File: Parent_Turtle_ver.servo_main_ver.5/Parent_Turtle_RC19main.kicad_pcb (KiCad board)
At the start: 2 copper layers, 70 x 60 mm, 61 parts, among them P1 CONN_02X15, P10 WRITING, P11 A/D, P12 5V_in, P13 CONN_02X04, P14 I/O, P15 CONN_02X04, P16 PWM, P17 SERIAL0, P2 CONN_02X15, P3 CAN, P4 CAN, P5 PWM, P6 SERIAL1, P7 SERIAL2, P8 WRITING_IN, P9 CAN_JP, Q1 NPN, SW1 SW1, SW2 SW0, U1 MAX3051, U2 MCP2221, U3 78L05

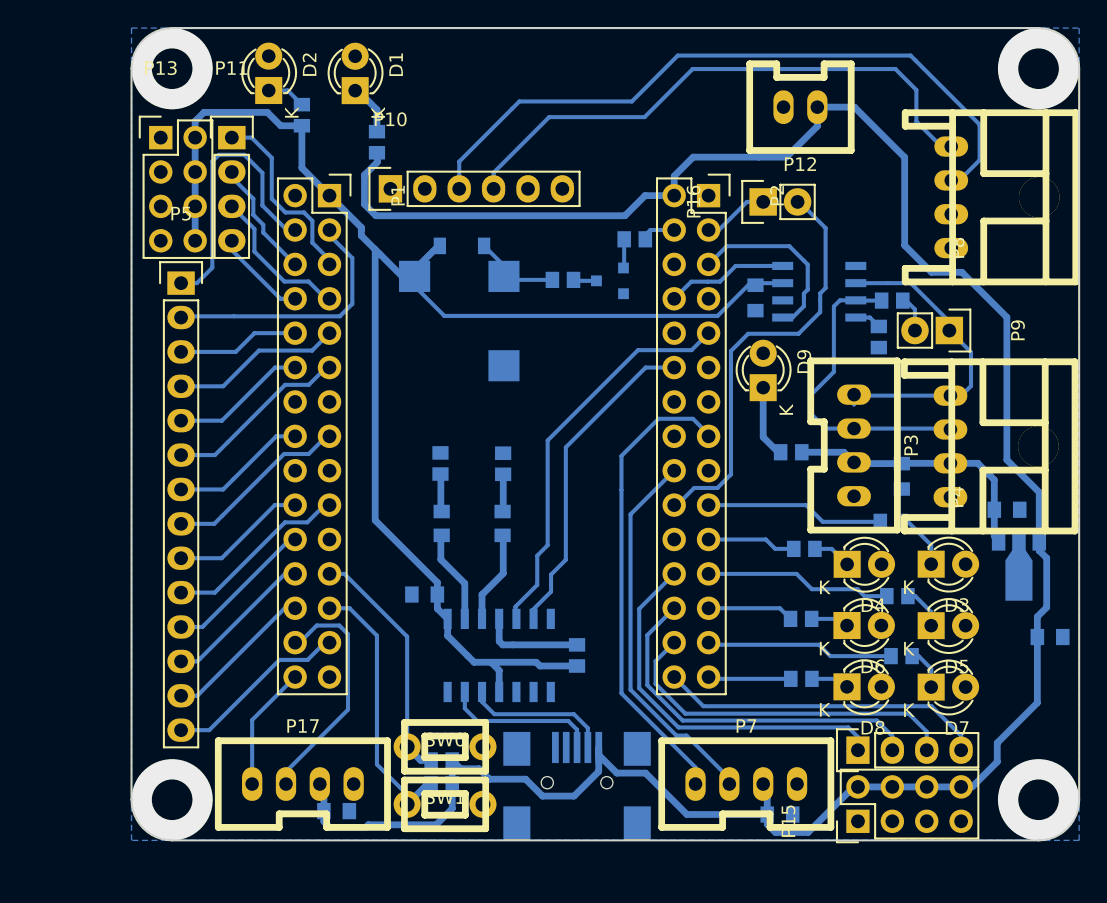
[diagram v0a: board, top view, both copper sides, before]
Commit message: クランリンケージ用main基板完成版
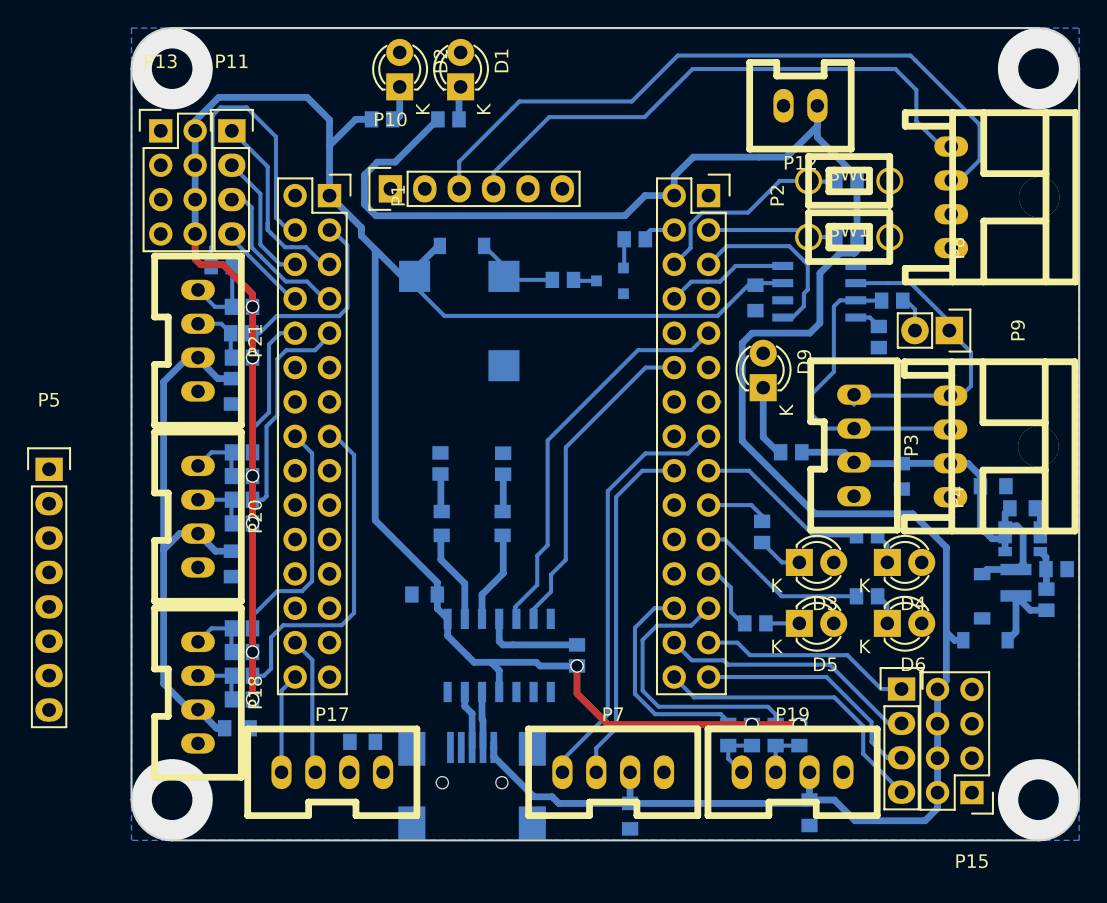
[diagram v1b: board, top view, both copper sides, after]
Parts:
- removed D7, D8: LED, LEDs:LED-3MM
- removed P16: PWM, Pin_Headers:Pin_Header_Straight_1x02
- removed R12, R13: 330, Resistors_SMD:R_0603
- added C10: 0.1u, Capacitors_SMD:C_0603, B.Cu at (108.5, 109.2)
- added C11: 0.1u, Capacitors_SMD:C_0603, B.Cu at (108.5, 96.5)
- added C8: 0.1u, Capacitors_SMD:C_0603, B.Cu at (151.2, 127.6)
- added C9: 0.1u, Capacitors_SMD:C_0603, B.Cu at (108.9, 121.4)
- added D13: DIODE, Mizz_lib:SOD-123, B.Cu at (163.9, 111.6)
- added D14: DIODE, Mizz_lib:SOD-123, B.Cu at (164.2, 114.9)
- added L1: 10uH, Inductors:Inductor_Wurth_MAPI-2512, B.Cu at (166.4, 110.6)
- added P18: ENC, RP_KiCAD_Connector:XA_4T, F.Cu at (106.0, 115.0)
- added P19: ENC, RP_KiCAD_Connector:XA_4T, F.Cu at (146.2, 124.6)
- added P20: ENC, RP_KiCAD_Connector:XA_4T, F.Cu at (106.0, 102.0)
- added P21: ENC, RP_KiCAD_Connector:XA_4T, F.Cu at (106.0, 89.0)
- added R19: 100, Resistors_SMD:R_0603, B.Cu at (109.2, 117.5)
- added R20: 100, Resistors_SMD:R_0603, B.Cu at (109.2, 114.0)
- added R21: 100, Resistors_SMD:R_0603, B.Cu at (148.7, 121.9)
- added R22: 100, Resistors_SMD:R_0603, B.Cu at (145.2, 121.9)
- added R23: 1k, Resistors_SMD:R_0603, B.Cu at (109.2, 119.2)
- added R24: 1k, Resistors_SMD:R_0603, B.Cu at (150.4, 121.9)
- added R25: 1k, Resistors_SMD:R_0603, B.Cu at (109.2, 115.8)
- added R26: 1k, Resistors_SMD:R_0603, B.Cu at (146.9, 121.9)
- added R27: 100, Resistors_SMD:R_0603, B.Cu at (109.2, 104.5)
- added R28: 100, Resistors_SMD:R_0603, B.Cu at (109.2, 101.0)
- added R29: 100, Resistors_SMD:R_0603, B.Cu at (109.2, 92.2)
- added R30: 100, Resistors_SMD:R_0603, B.Cu at (107.8, 87.2)
- added R31: 1k, Resistors_SMD:R_0603, B.Cu at (109.2, 106.2)
- added R32: 1k, Resistors_SMD:R_0603, B.Cu at (109.2, 94.0)
- added R33: 1k, Resistors_SMD:R_0603, B.Cu at (109.2, 102.8)
- added R34: 1k, Resistors_SMD:R_0603, B.Cu at (109.2, 90.2)
- added R35: 50k, Resistors_SMD:R_0603, B.Cu at (168.7, 111.9)
- added R36: 10k, Resistors_SMD:R_0603, B.Cu at (169.4, 109.6)
- C7: value 0.1u -> 1u
- P11: value A/D -> ADC
- P13: value CONN_02X04 -> ADC/Vdd/GND
- P15: value CONN_02X04 -> I/O /Vdd/GND
- P5: footprint Pin_Headers:Pin_Header_Straight_1x14 -> Pin_Headers:Pin_Header_Straight_1x08
- U3: value 78L05 -> AOZ1280; footprint TO_SOT_Packages_SMD:SOT89-3_Housing -> Mizz_lib:TSOT-6-MK06A
- moved R7 52.2 mm to (153.9, 81.0)
- moved SW1 51.4 mm to (154.1, 85.1)
- moved SW2 51.4 mm to (154.1, 81.0)
- moved R2 50.3 mm to (153.9, 85.1)
- moved P5 16.9 mm to (95.0, 102.2)
- moved C7 11.9 mm to (164.8, 103.5)
- moved C3 11.1 mm to (137.9, 127.9), turned to 270 degrees
- moved R10 10.7 mm to (147.2, 113.6)
- moved P7 9.87 mm to (132.9, 124.6)
- moved D5 9.74 mm to (150.4, 113.6)
- moved D3 9.74 mm to (150.4, 109.1)
- moved D2 9.68 mm to (120.9, 74.0)
- moved R3 9.54 mm to (147.7, 106.9), turned to 270 degrees
- moved P15 8.68 mm to (163.2, 126.1), turned to 180 degrees
- moved D1 7.80 mm to (125.4, 74.0)
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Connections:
- C6 pad 1: +12V -> Net-(C6-Pad1)
- C6 pad 2: GND -> Net-(C6-Pad2)
- C7 pad 1: +5V -> +12V
- P14 pad 1: /D15 -> /D8
- P14 pad 2: /D13 -> /D9
- P14 pad 3: /D9 -> /B15
- P5 pad 1: /E6 -> Net-(P5-Pad1)
- P5 pad 2: /E5 -> Net-(P5-Pad2)
- P5 pad 3: /A1 -> Net-(P5-Pad3)
- P5 pad 4: /A0 -> Net-(P5-Pad4)
- P5 pad 5: /A3 -> Net-(P5-Pad5)
- P5 pad 6: /A2 -> Net-(P5-Pad6)
- P5 pad 7: /A7 -> Net-(P5-Pad7)
- P5 pad 8: /A6 -> Net-(P5-Pad8)
- R11 pad 1: /D12 -> /C6
- R2 pad 2: /E12 -> /B8
- R4 pad 1: /C6 -> /A8
- R7 pad 2: /E10 -> /B7
- SW1 pad 2: /E12 -> /B8
- SW2 pad 2: /E10 -> /B7
- U3 pad 1: +12V -> Net-(C6-Pad2)
- U3 pad 3: +5V -> /FB
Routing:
- net +3.3V: track 109.5 -> 172.5 mm, vias 0 -> 9
- net /C9: track 31.3 -> 0.00 mm
- net +5V: track 171.7 -> 201.8 mm
- net /D15: track 28.2 -> 0.00 mm
- net /E12: track 20.1 -> 0.00 mm
- net /E10: track 18.0 -> 0.00 mm
- net /B7: track 0.00 -> 15.6 mm
- net /D12: track 6.38 -> 20.9 mm
- net /A2: track 13.6 -> 0.25 mm
- net /E14: track 13.6 -> 0.34 mm
- net /B0: track 13.6 -> 0.36 mm
- net /A8: track 0.00 -> 12.9 mm
- net /B15: track 6.13 -> 17.6 mm
- net /A6: track 13.6 -> 24.8 mm
- net /E13: track 11.1 -> 0.00 mm
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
